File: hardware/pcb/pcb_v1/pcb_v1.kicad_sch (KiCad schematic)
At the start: 26 parts, among them J1 Conn_01x10, J2 Conn_01x10, J3 Conn_01x10, J4 Conn_01x10, U1 Pico, U3 TL2575-05

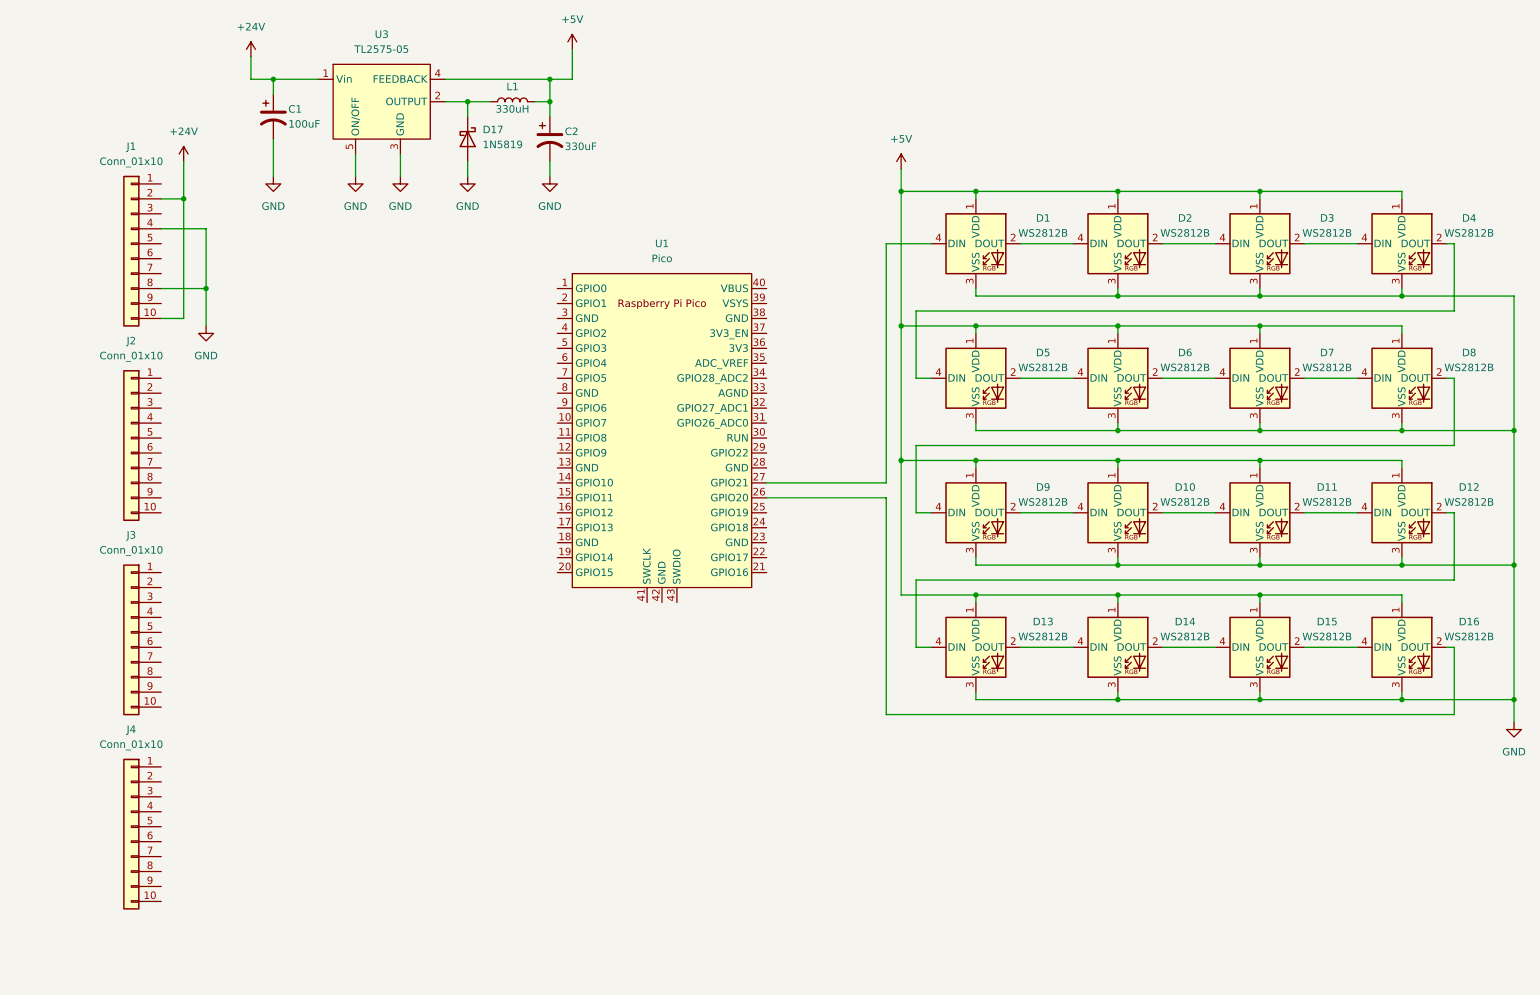
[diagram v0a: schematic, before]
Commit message: worked on pcbv1
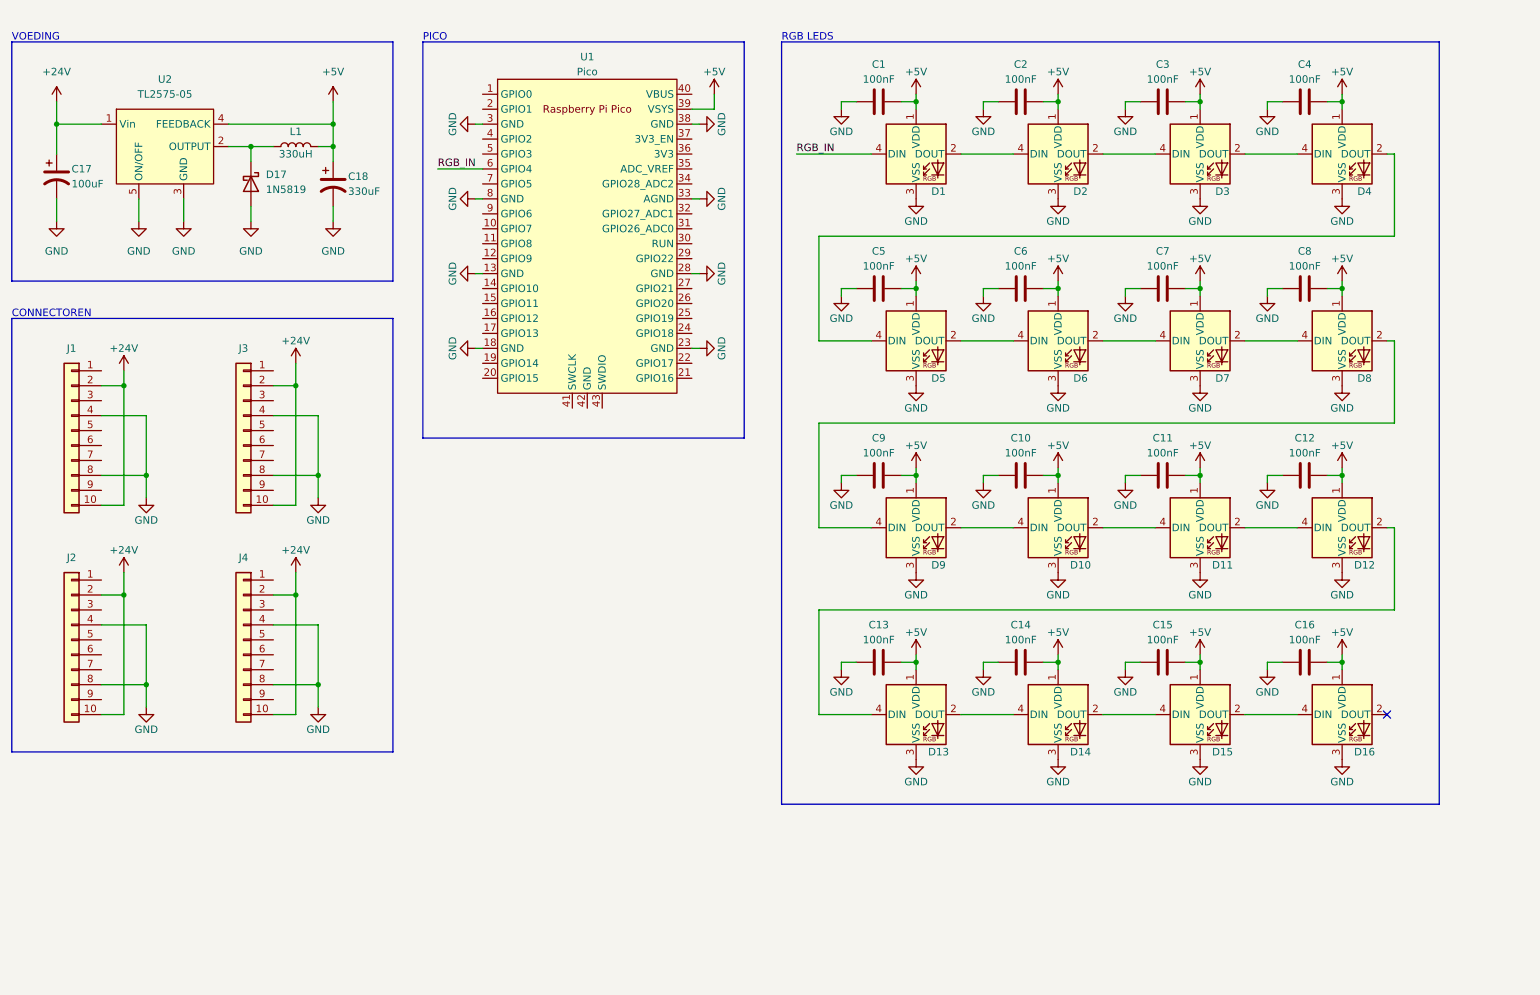
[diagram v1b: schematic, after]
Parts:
- added C1, C10, C11, C12, C13, C14, C15, C16, C2, C3, C4, C5, C6, C7, C8, C9: 100nF, Capacitor_SMD:C_0805_2012Metric, symbol Device:C
- C17: renamed from C1; footprint (none) -> Capacitor_SMD:CP_Elec_8x10
- C18: renamed from C2; footprint (none) -> Capacitor_SMD:CP_Elec_10x10
- L1: footprint (none) -> Inductor_SMD:L_12x12mm_H8mm
- U2: renamed from U3; footprint (none) -> Package_TO_SOT_SMD:TO-263-5_TabPin3
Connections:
- net +24V: now also J2.10 (Pin_10), J2.2 (Pin_2), J3.10 (Pin_10), J3.2 (Pin_2), J4.10 (Pin_10), J4.2 (Pin_2)
- net +5V: now also U1.39 (VSYS), C1.2, C10.2, C11.2, C12.2, C13.2, C14.2, C15.2, C16.2, C2.2, C3.2, C4.2, C5.2, C6.2, C7.2, C8.2, C9.2
- net GND: now also J2.4 (Pin_4), J2.8 (Pin_8), J3.4 (Pin_4), J3.8 (Pin_8), J4.4 (Pin_4), J4.8 (Pin_8), U1.13 (GND), U1.18 (GND), U1.23 (GND), U1.28 (GND), U1.3 (GND), U1.33 (AGND), U1.38 (GND), U1.8 (GND), C1.1, C10.1, C11.1, C12.1, C13.1, C14.1, C15.1, C16.1, C2.1, C3.1, C4.1, C5.1, C6.1, C7.1, C8.1, C9.1
- net at D16.2 (DOUT): no longer U1.26 (GPIO20)
- net at U1.27 (GPIO21): no longer D1.4 (DIN)
- net RGB_IN: now reaches U1.6 (GPIO4)
- net RGB_IN: now also D1.4 (DIN)
- no-connect marks 0 -> 1
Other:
- note added: "CONNECTOREN"
- note added: "PICO"
- note added: "RGB LEDS"
- note added: "VOEDING"
- moved on the sheet: C17, C18, D1, D10, D11, D12, D13, D14, D15, D16, D17, D2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

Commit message: finished pcbv1
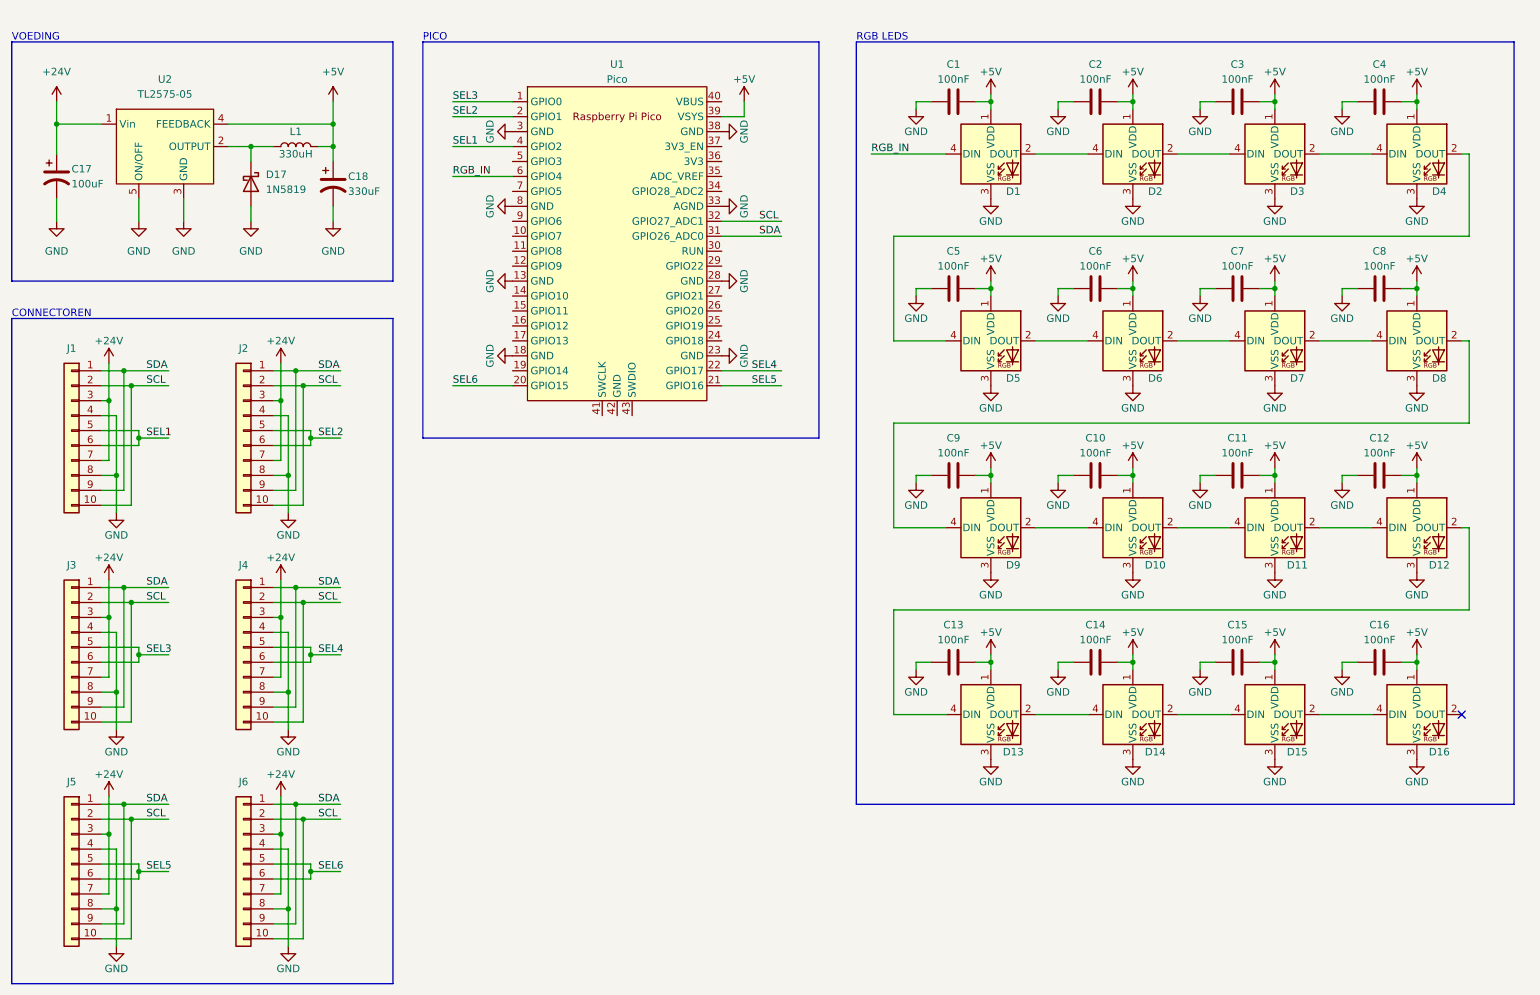
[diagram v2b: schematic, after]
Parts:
- added J5, J6: Conn_01x10, Connector_PinHeader_2.54mm:PinHeader_2x05_P2.54mm_Vertical, symbol Connector_Generic:Conn_01x10
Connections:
- net +24V: now also J1.3 (Pin_3), J1.7 (Pin_7), J2.3 (Pin_3), J2.7 (Pin_7), J3.3 (Pin_3), J3.7 (Pin_7), J4.3 (Pin_3), J4.7 (Pin_7), J5.3 (Pin_3), J5.7 (Pin_7), J6.3 (Pin_3), J6.7 (Pin_7); no longer J1.10 (Pin_10), J1.2 (Pin_2), J2.10 (Pin_10), J2.2 (Pin_2), J3.10 (Pin_10), J3.2 (Pin_2), J4.10 (Pin_10), J4.2 (Pin_2)
- net GND: now also J5.4 (Pin_4), J5.8 (Pin_8), J6.4 (Pin_4), J6.8 (Pin_8)
- net SDA: now reaches J1.1 (Pin_1)
- net SDA: now also J1.9 (Pin_9), J2.1 (Pin_1), J2.9 (Pin_9), J3.1 (Pin_1), J3.9 (Pin_9), J4.1 (Pin_1), J4.9 (Pin_9), U1.31 (GPIO26_ADC0), J5.1 (Pin_1), J5.9 (Pin_9), J6.1 (Pin_1), J6.9 (Pin_9)
- net SEL1: now reaches J1.5 (Pin_5)
- net SEL1: now also J1.6 (Pin_6), U1.4 (GPIO2)
- net SEL3: now reaches U1.1 (GPIO0)
- net SEL3: now also J3.5 (Pin_5), J3.6 (Pin_6)
- net SEL2: now reaches U1.2 (GPIO1)
- net SEL2: now also J2.5 (Pin_5), J2.6 (Pin_6)
- net SEL6: now reaches U1.20 (GPIO15)
- net SEL6: now also J6.5 (Pin_5), J6.6 (Pin_6)
- net SEL5: now reaches U1.21 (GPIO16)
- net SEL5: now also J5.5 (Pin_5), J5.6 (Pin_6)
- net SEL4: now reaches U1.22 (GPIO17)
- net SEL4: now also J4.5 (Pin_5), J4.6 (Pin_6)
- net SCL: now reaches U1.32 (GPIO27_ADC1)
- net SCL: now also J1.10 (Pin_10), J1.2 (Pin_2), J2.10 (Pin_10), J2.2 (Pin_2), J3.10 (Pin_10), J3.2 (Pin_2), J4.10 (Pin_10), J4.2 (Pin_2), J5.10 (Pin_10), J5.2 (Pin_2), J6.10 (Pin_10), J6.2 (Pin_2)
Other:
- title: (none) -> Lannooleaf PCB schema
- moved on the sheet: C1, C10, C11, C12, C13, C14, C15, C16, C2, C3, C4, C5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
